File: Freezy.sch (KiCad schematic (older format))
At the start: 5 parts, among them CON501 AVR-ISP-6, IC501 ATTINY25-SS, P501 CONN_01X02

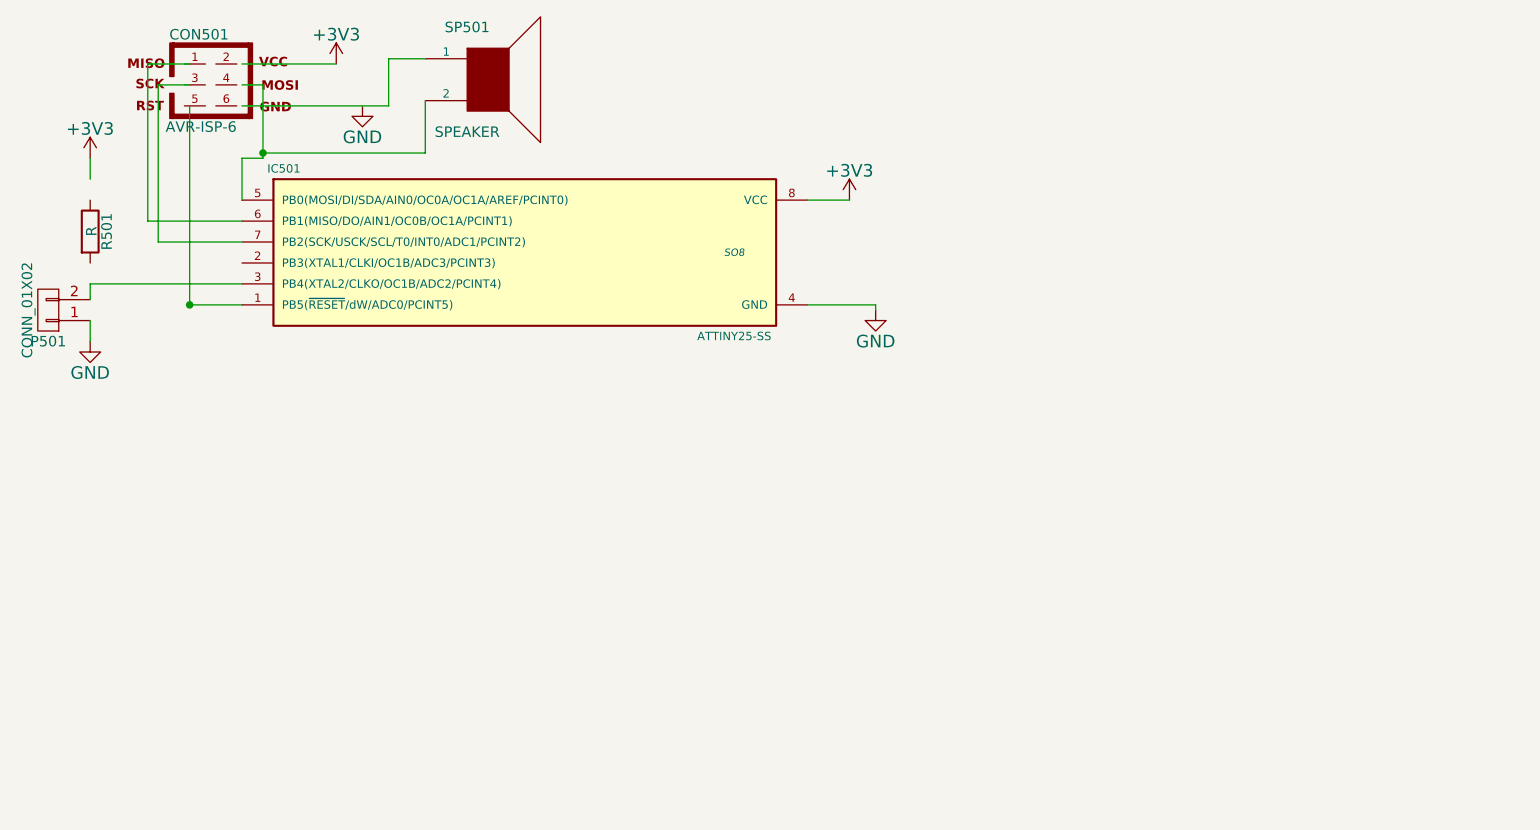
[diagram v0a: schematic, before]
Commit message: Version 0.2
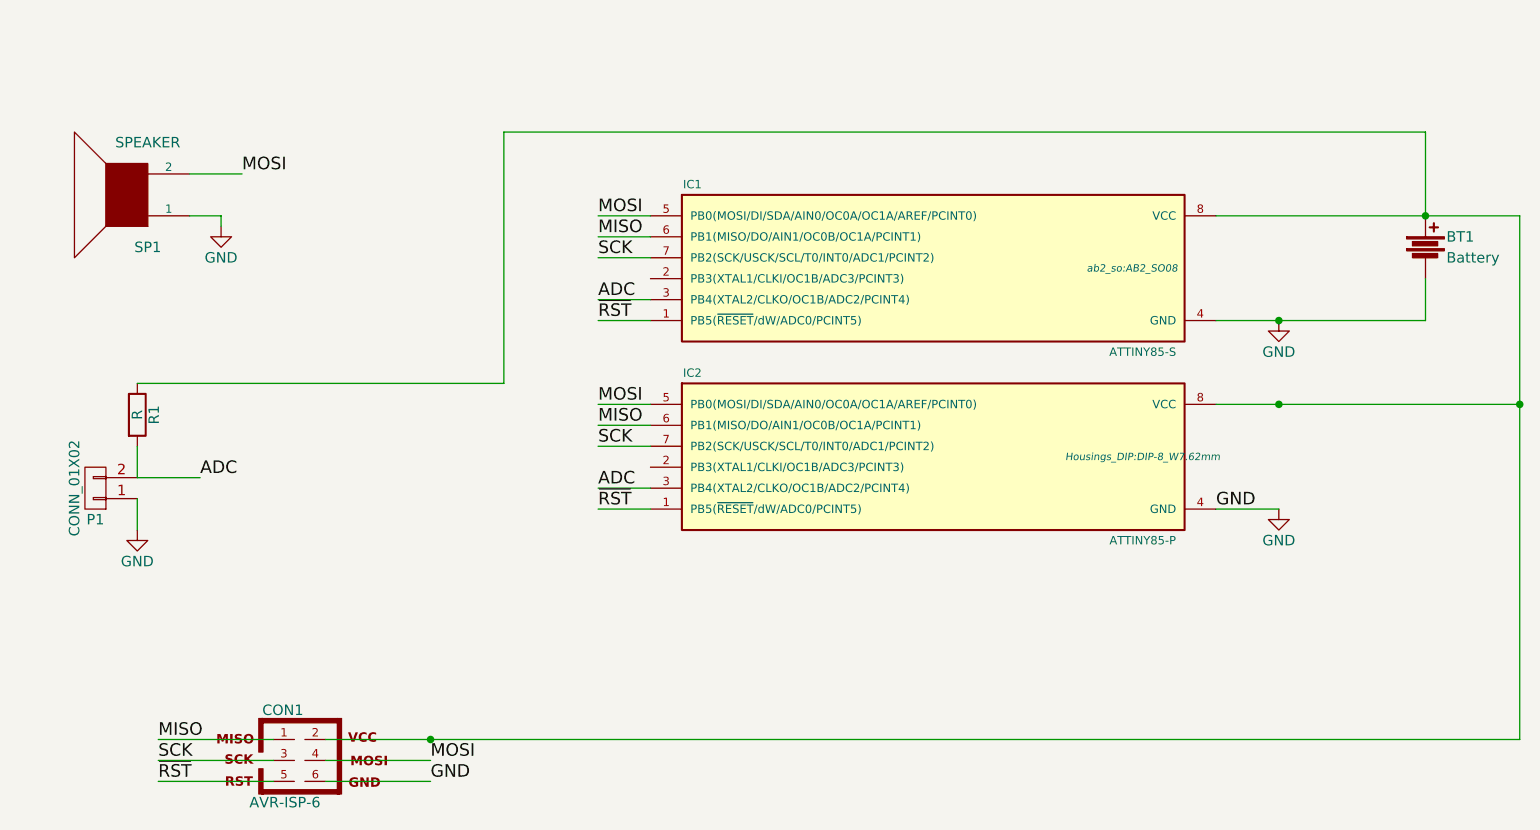
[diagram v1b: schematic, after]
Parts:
- removed CON501: AVR-ISP-6, AVR-ISP-6, symbol AVR-ISP-6
- removed IC501: ATTINY25-SS, SO8, symbol ATTINY25-SS
- removed P501: CONN_01X02, symbol CONN_01X02
- removed R501: R, symbol R
- removed SP501: SPEAKER, symbol SPEAKER
- added BT1: Battery, Pin_Headers:Pin_Header_Straight_1x01, symbol Battery
- added CON1: AVR-ISP-6, Pin_Headers:Pin_Header_Straight_2x03, symbol AVR-ISP-6
- added IC1: ATTINY85-S, ab2_so:AB2_SO08, symbol ATTINY85-S
- added IC2: ATTINY85-P, Housings_DIP:DIP-8_W7.62mm, symbol ATTINY85-P
- added P1: CONN_01X02, Pin_Headers:Pin_Header_Straight_1x02, symbol CONN_01X02
- added R1: R, Resistors_SMD:R_0805, symbol R
- added SP1: SPEAKER, footprints:buzzer, symbol SPEAKER
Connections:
- net labels added: ADC, MISO, MOSI, SCK, ~RST
- net labels removed: +3V3
- wire segments 25 -> 32
